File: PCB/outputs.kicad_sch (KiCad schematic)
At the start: 8 parts, among them J10 FINAL_CARRERA, J12 DOOR_LCK, J13 WIN_SW, J2 OUT_WIN, J5 OUT_DOOR, J6 UART, J7 SPI, J9 CAN

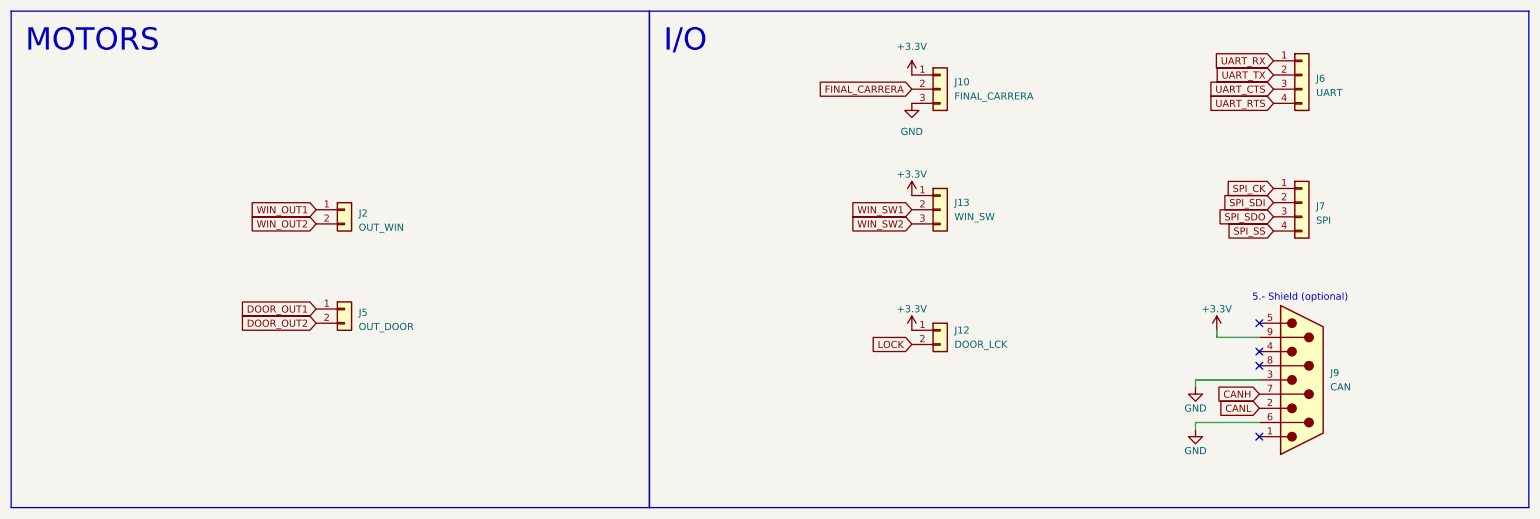
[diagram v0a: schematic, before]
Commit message: sparse changes
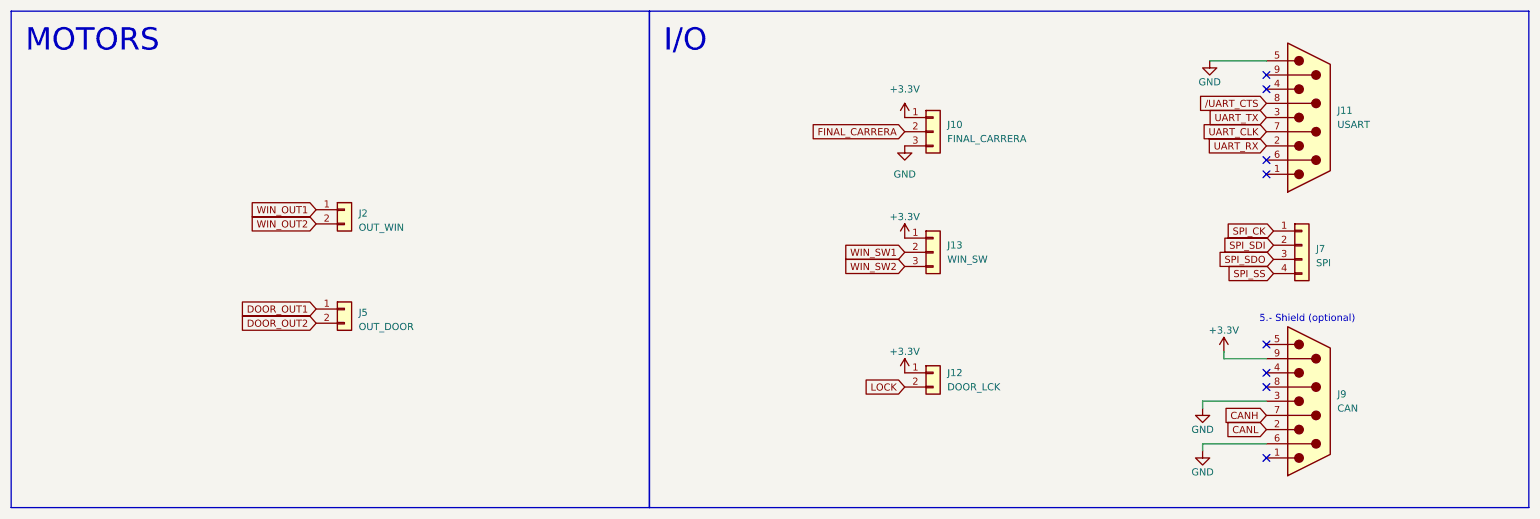
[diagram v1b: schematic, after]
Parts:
- removed J6: UART, symbol Connector_Generic:Conn_01x04
- added J11: USART, symbol Connector:DE9_Plug
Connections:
- net GND: now also J11.5
- net UART_RX: now also J11.2
- net UART_TX: now also J11.3
- new net UART_CLK: J11.7
- new net /UART_CTS: J11.8
- no-connect marks 4 -> 8
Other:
- moved on the sheet: J10, J12, J13, J7, J9
